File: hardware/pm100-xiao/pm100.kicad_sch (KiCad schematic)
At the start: 44 parts, among them J1 VCC-BATT, J2 VCC-ESC, J4 GND-BATT, J5 UART, J6 RECEIVER, J7 ESC, J8 SAFETY, Q5 BSS138, Q6 BSS138, Q7 BSS138, Q8 BSS138, Q9 BSS138, U2 LMR16006YQ5, U8 INA226

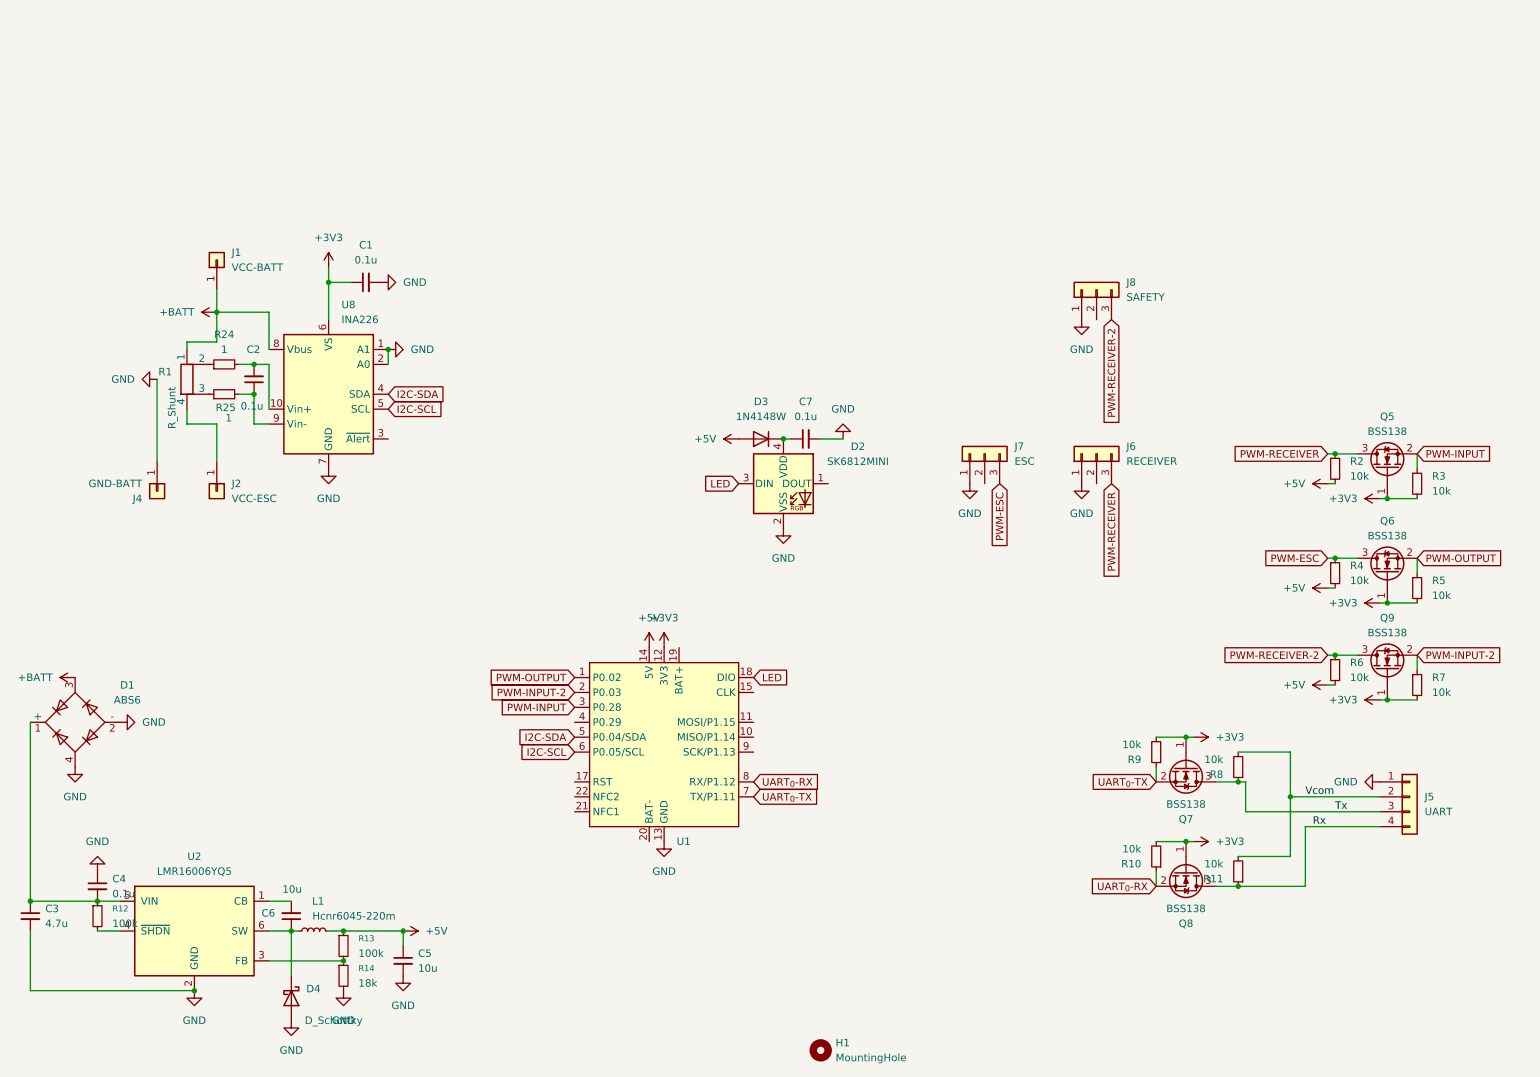
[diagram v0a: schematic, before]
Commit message: rev4 projeto eletronico
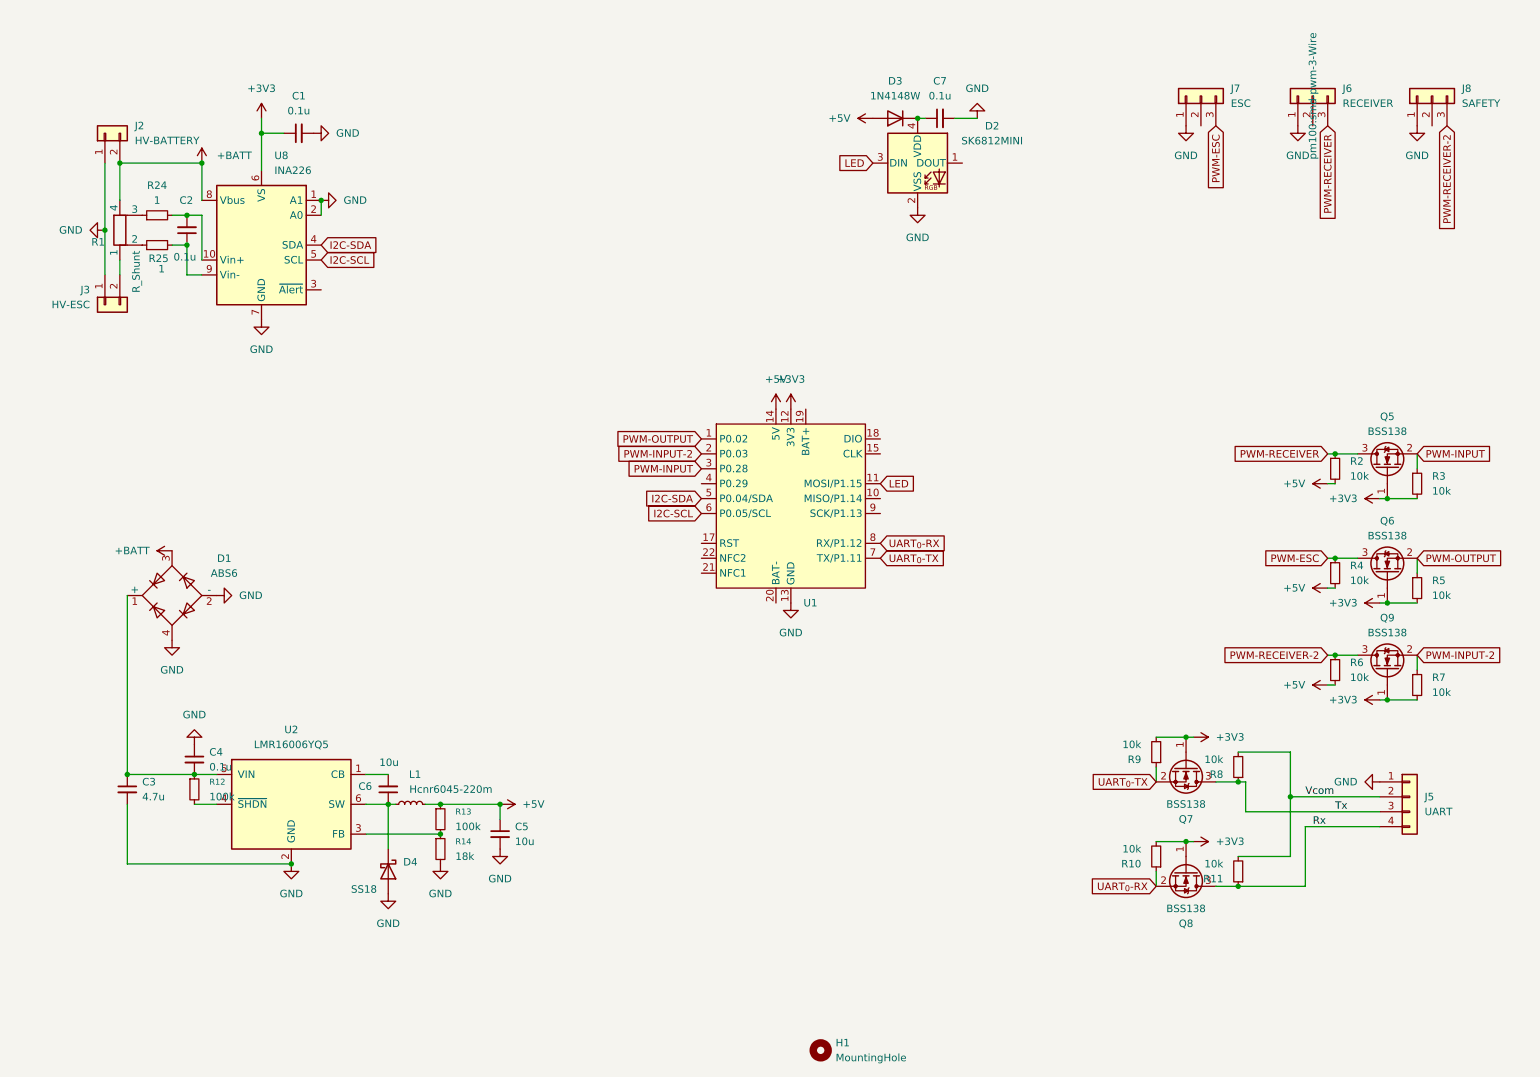
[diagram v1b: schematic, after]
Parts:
- removed J1: VCC-BATT, footprints:HV_CONN_01x01_pad_6.2x12mm, symbol Connector_Generic:Conn_01x01
- removed J2: VCC-ESC, footprints:HV_CONN_01x01_pad_6.2x12mm, symbol Connector_Generic:Conn_01x01
- removed J4: GND-BATT, footprints:HV_CONN_01x01_pad_6.2x12mm, symbol Connector_Generic:Conn_01x01
- added J2: HV-BATTERY, Connector_AMASS:AMASS_XT60IPW-M_1x03_P7.20mm_Horizontal, symbol Connector_Generic:Conn_01x02
- added J3: HV-ESC, Connector_AMASS:AMASS_XT60PW-F_1x02_P7.20mm_Horizontal, symbol Connector_Generic:Conn_01x02
- D4: value D_Schottky -> SS18
- J5: footprint Connector_JST:JST_XH_S4B-XH-A-1_1x04_P2.50mm_Horizontal -> Connector_Hirose:Hirose_DF13-04P-1.25DS_1x04_P1.25mm_Horizontal
- J6, J7, J8: footprint Sigma Footprints:SolderWire_SMD_3 -> pm100:smd-pwm-3-Wire
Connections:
- net +BATT: now also R1.4, J2.2 (Pin_2); no longer R1.1
- net GND: now also J2.1 (Pin_1), J3.1 (Pin_1)
- net LED: now also U1.11 (MOSI/P1.15); no longer U1.18 (DIO)
- net at R24.1: now also R1.3; no longer R1.2
- net at R25.1: now also R1.2; no longer R1.3
- new net: J3.2 (Pin_2), R1.1
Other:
- moved on the sheet: C1, C2, C3, C4, C5, C6, C7, D1, D2, D3, D4, J6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
